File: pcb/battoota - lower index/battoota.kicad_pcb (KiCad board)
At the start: 2 copper layers, 124.7 x 97.3 mm, 38 parts

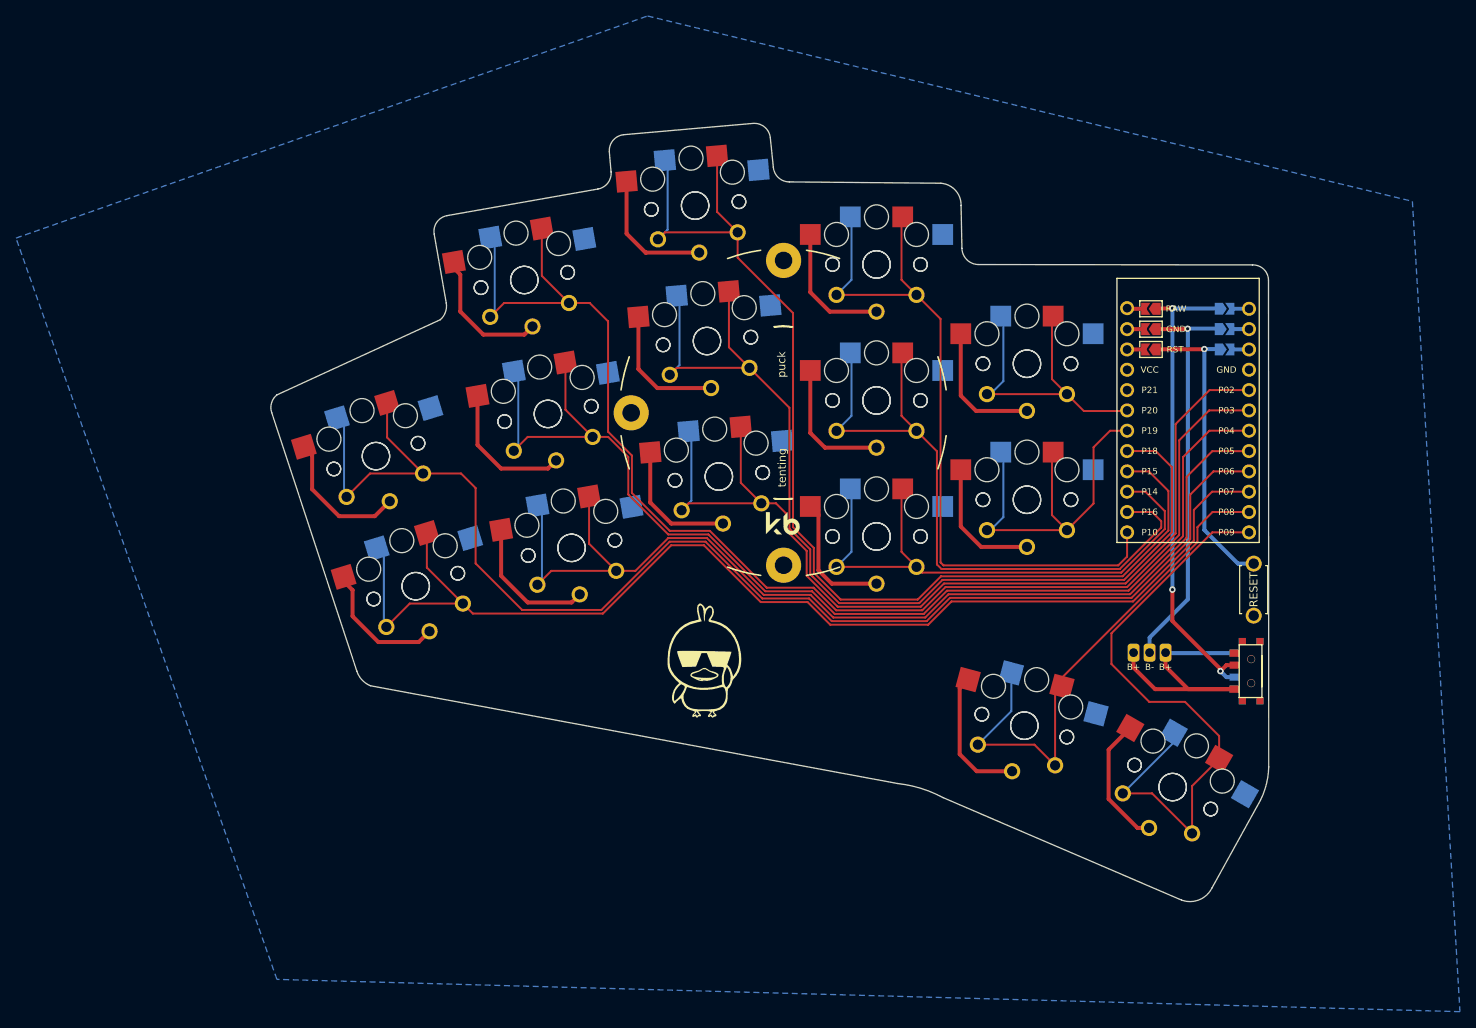
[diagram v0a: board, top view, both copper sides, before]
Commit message: pcb shape change
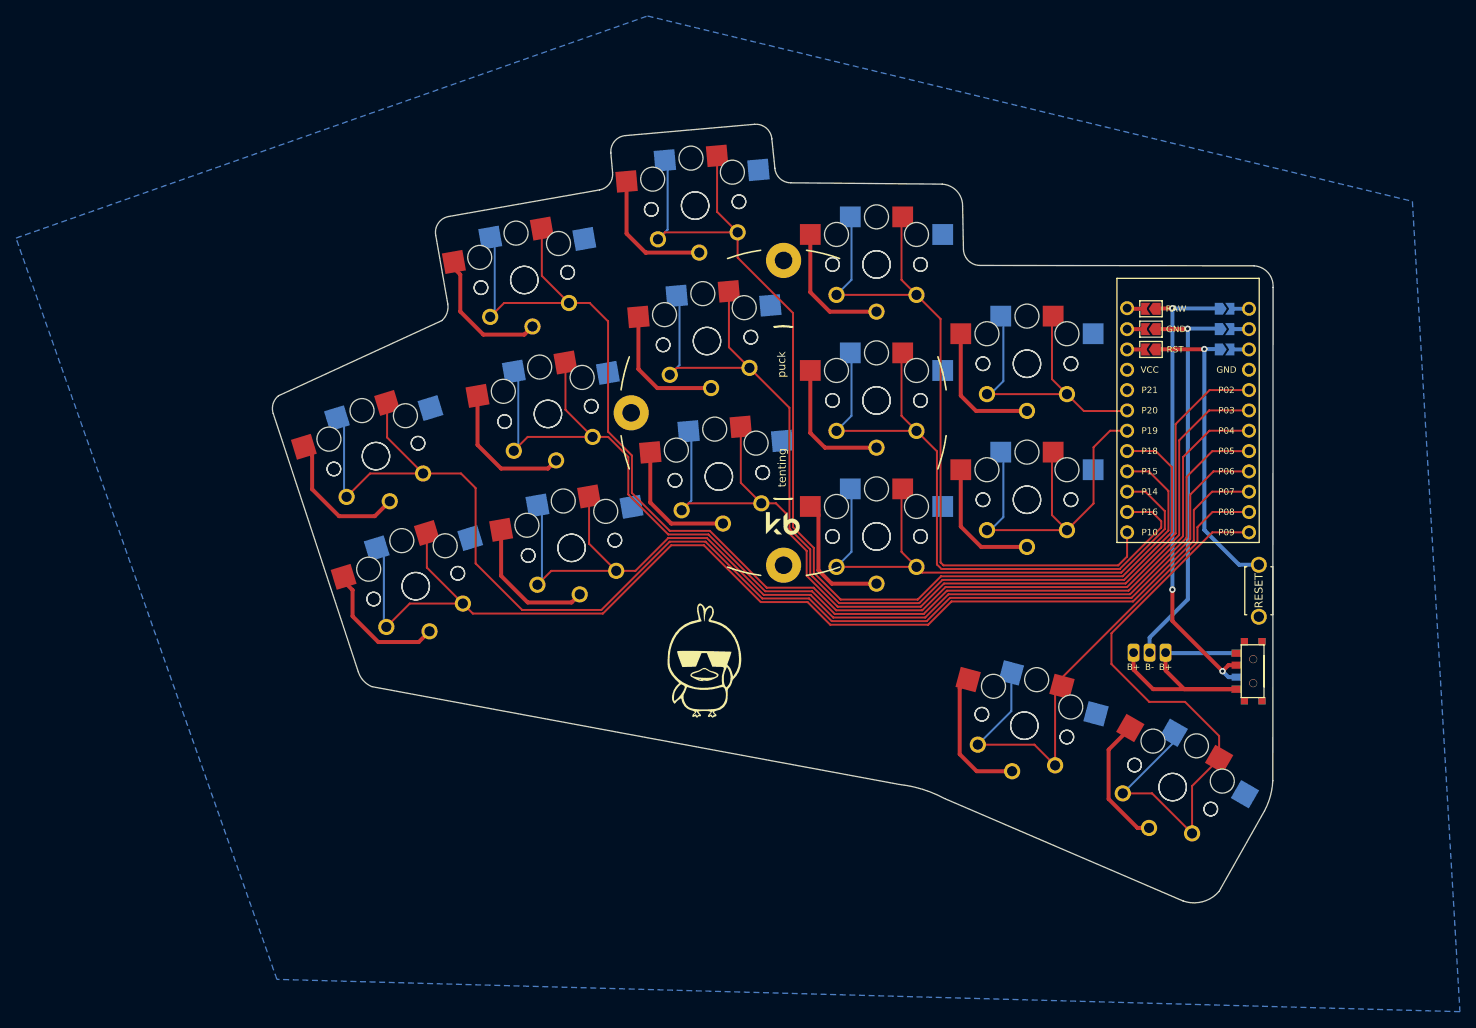
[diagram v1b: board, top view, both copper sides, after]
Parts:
- moved B1 0.66 mm to (163.2, -65.9)
- moved T1 0.26 mm to (162.5, -55.8)
- moved T2 0.26 mm to (162.5, -55.8)
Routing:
- net Braw: track 35.8 -> 37.0 mm
- net RST: track 38.3 -> 39.0 mm
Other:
- board size 124.7 x 97.3 mm -> 125.1 x 97.3 mm
